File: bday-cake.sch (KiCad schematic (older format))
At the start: 3 parts

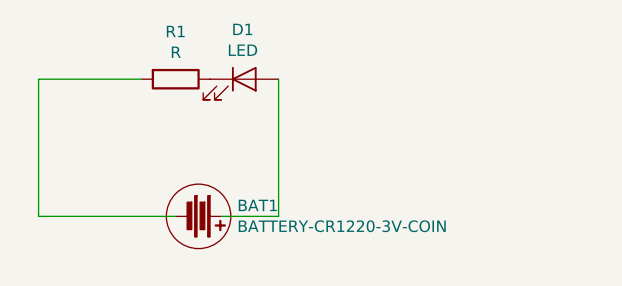
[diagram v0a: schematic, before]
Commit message: update layout
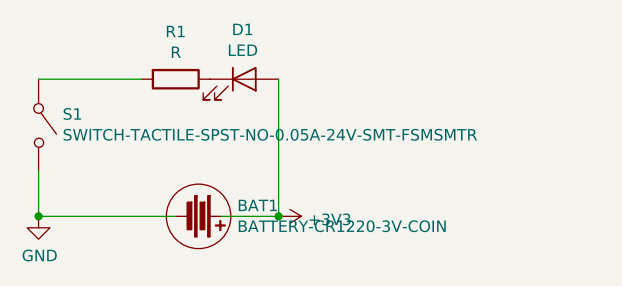
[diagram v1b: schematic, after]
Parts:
- added S1: SWITCH-TACTILE-SPST-NO-0.05A-24V-SMT-FSMSMTR, Wickerlib:SWITCH-TECONN-MOMENTARY-SMD-FSMSM, symbol wickerlib:SWITCH-TACTILE-SPST-NO-0.05A-24V-SMT-FSMSMTR
- R1: footprint Resistor_THT:R_Axial_DIN0207_L6.3mm_D2.5mm_P2.54mm_Vertical -> Resistor_THT:R_Axial_DIN0207_L6.3mm_D2.5mm_P7.62mm_Horizontal
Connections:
- net labels added: +3V3, GND
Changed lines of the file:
@@
 F 0 "R1" V 4993 2200 50  0000 C CNN
 F 1 "R" V 5084 2200 50  0000 C CNN
-F 2 "Resistor_THT:R_Axial_DIN0207_L6.3mm_D2.5mm_P2.54mm_Vertical" V 5130 2200 50  0001 C CNN
+F 2 "Resistor_THT:R_Axial_DIN0207_L6.3mm_D2.5mm_P7.62mm_Horizontal" V 5130 2200 50  0001 C CNN
 F 3 "~" H 5200 2200 50  0001 C CNN
 	1    5200 2200
@@
 	5050 2200 4600 2200
 Wire Wire Line
-	4600 2200 4600 2800
+	5650 2800 5650 2200
 Wire Wire Line
-	4600 2800 5200 2800
+	5200 2800 4600 2800
 Wire Wire Line
 	5400 2800 5650 2800
+$Comp
+L power:GND #PWR0101
+U 1 1 5E264F45
+P 4600 2800
+F 0 "#PWR0101" H 4600 2550 50  0001 C CNN
+F 1 "GND" H 4605 2627 50  0000 C CNN
+F 2 "" H 4600 2800 50  0001 C CNN
+F 3 "" H 4600 2800 50  0001 C CNN
+	1    4600 2800
+	1    0    0    -1
+$EndComp
+$Comp
+L power:+3V3 #PWR0102
+U 1 1 5E266A09
+P 5650 2800
+F 0 "#PWR0102" H 5650 2650 50  0001 C CNN
+F 1 "+3V3" V 5665 2928 50  0000 L CNN
+F 2 "" H 5650 2800 50  0001 C CNN
+F 3 "" H 5650 2800 50  0001 C CNN
+	1    5650 2800
+	0    1    1    0
+$EndComp
+Connection ~ 5650 2800
+$Comp
+L wickerlib:SWITCH-TACTILE-SPST-NO-0.05A-24V-SMT-FSMSMTR S1
+U 1 1 5E26A03A
+P 4600 2450
+F 0 "S1" V 4504 2555 50  0000 L CNN
+F 1 "SWITCH-TACTILE-SPST-NO-0.05A-24V-SMT-FSMSMTR" V 4595 2555 50  0000 L CNN
+F 2 "Wickerlib:SWITCH-TECONN-MOMENTARY-SMD-FSMSM" H 4600 2100 50  0001 C CIN
+F 3 "http://www.te.com/commerce/DocumentDelivery/DDEController?Action=srchrtrv&DocNm=1437566-3&DocType=Customer+Drawing&DocLang=English" H 4600 2450 5   0001 C CNN
+F 4 "SWITCH TACTILE SPST-NO 0.05A 24V" H 4600 2100 50  0001 C CIN "Description"
+F 5 "TE Conn" H 4600 2100 50  0001 C CIN "MF_Name"
+F 6 "FSMSMTR" H 4600 2100 50  0001 C CIN "MF_PN"
+F 7 "Digikey" H 4600 2100 50  0001 C CIN "S1_Name"
+F 8 "450-1758-1-ND" H 4600 2100 50  0001 C CIN "S1_PN"
+F 9 "461" H 4600 2100 50  0001 C CIN "XSize_mils"
+F 10 "154" H 4600 2100 50  0001 C CIN "YSize_mils"
+F 11 "smt" H 4600 2100 50  0001 C CIN "Type"
+	1    4600 2450
+	0    1    1    0
+$EndComp
 Wire Wire Line
-	5650 2800 5650 2200
+	4600 2600 4600 2800
+Connection ~ 4600 2800
 $EndSCHEMATC
